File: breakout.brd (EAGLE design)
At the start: 50 x 50 mm, 33 parts

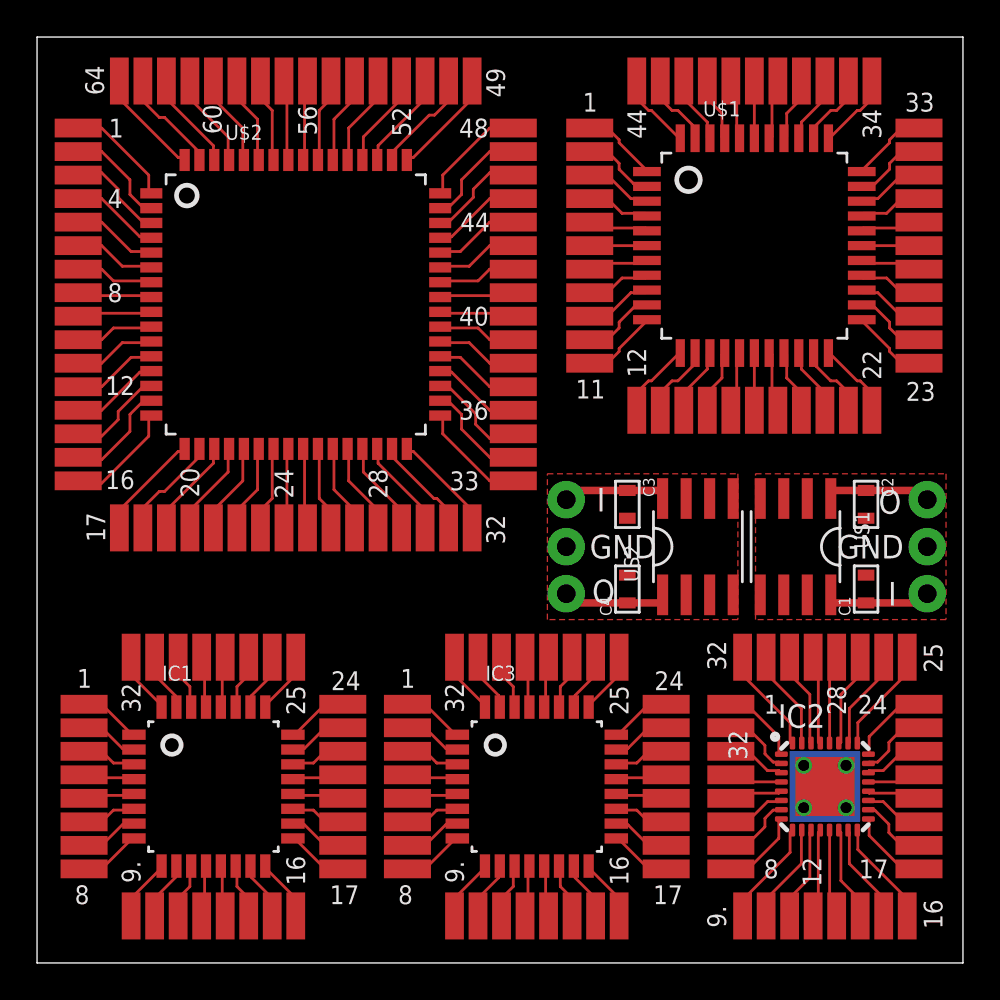
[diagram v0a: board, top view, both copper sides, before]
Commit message: Minor corrections. Ready to send.
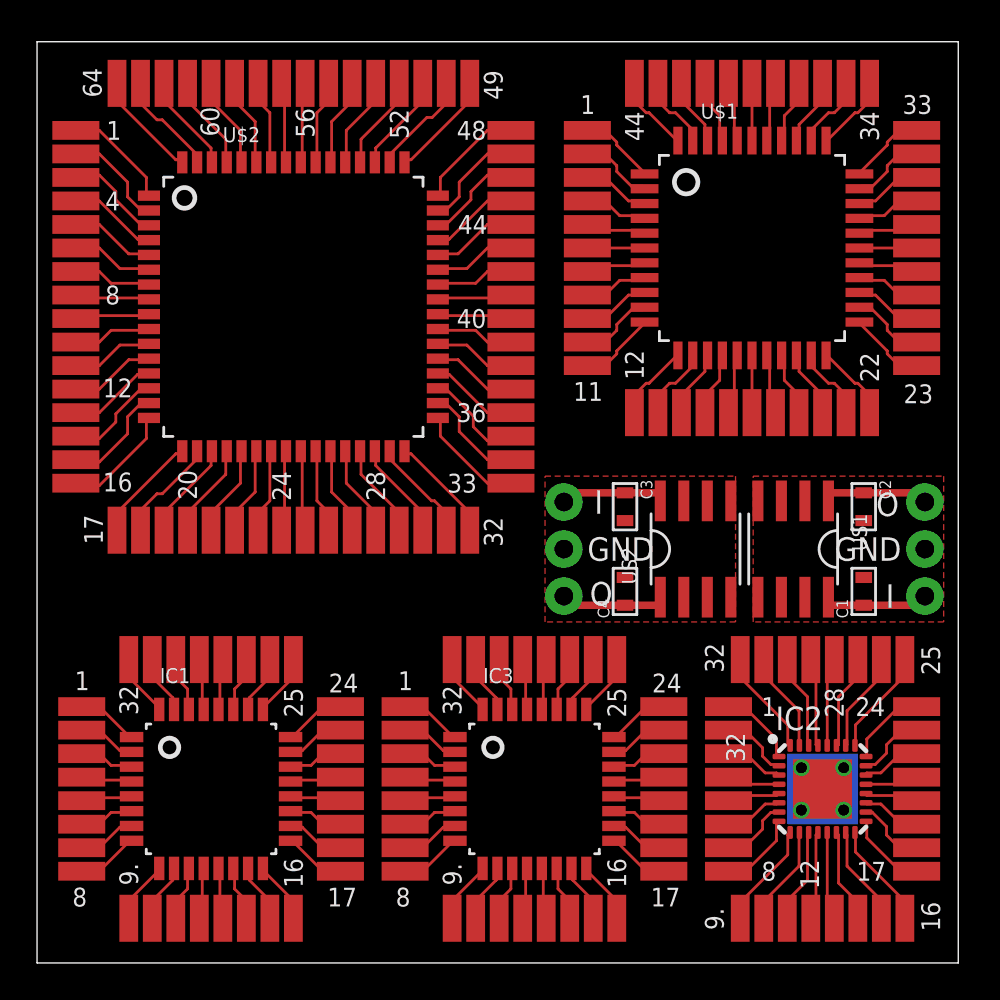
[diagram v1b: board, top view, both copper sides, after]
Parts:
- moved CON11 0.18 mm to (25.6, 35.4)
- moved CON16 0.18 mm to (42.4, 16.4)
- moved CON21 0.18 mm to (26.9, 16.4)
- moved CON7 0.18 mm to (47.5, 38.6)
- moved CON8 0.18 mm to (38.6, 47.5)
- moved U$1 0.18 mm to (38.6, 38.6)
- moved CON10 0.18 mm to (13.8, 23.4)
- moved CON12 0.18 mm to (13.8, 47.5)
- moved CON13 0.18 mm to (37.3, 9.40)
- moved CON15 0.18 mm to (47.5, 9.40)
- moved CON18 0.18 mm to (19.9, 9.40)
- moved CON3 0.18 mm to (16.4, 9.40)
- moved CON4 0.18 mm to (9.40, 16.4)
- moved IC2 0.18 mm to (42.4, 9.40)
- moved IC3 0.18 mm to (26.9, 9.40)
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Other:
- board size 50 x 50 mm -> 49.7 x 49.7 mm
